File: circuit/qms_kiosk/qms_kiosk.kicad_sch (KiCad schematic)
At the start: 3 parts, among them U1 LCD2X16, U2 CEG003400, U3 ESP32-CAM

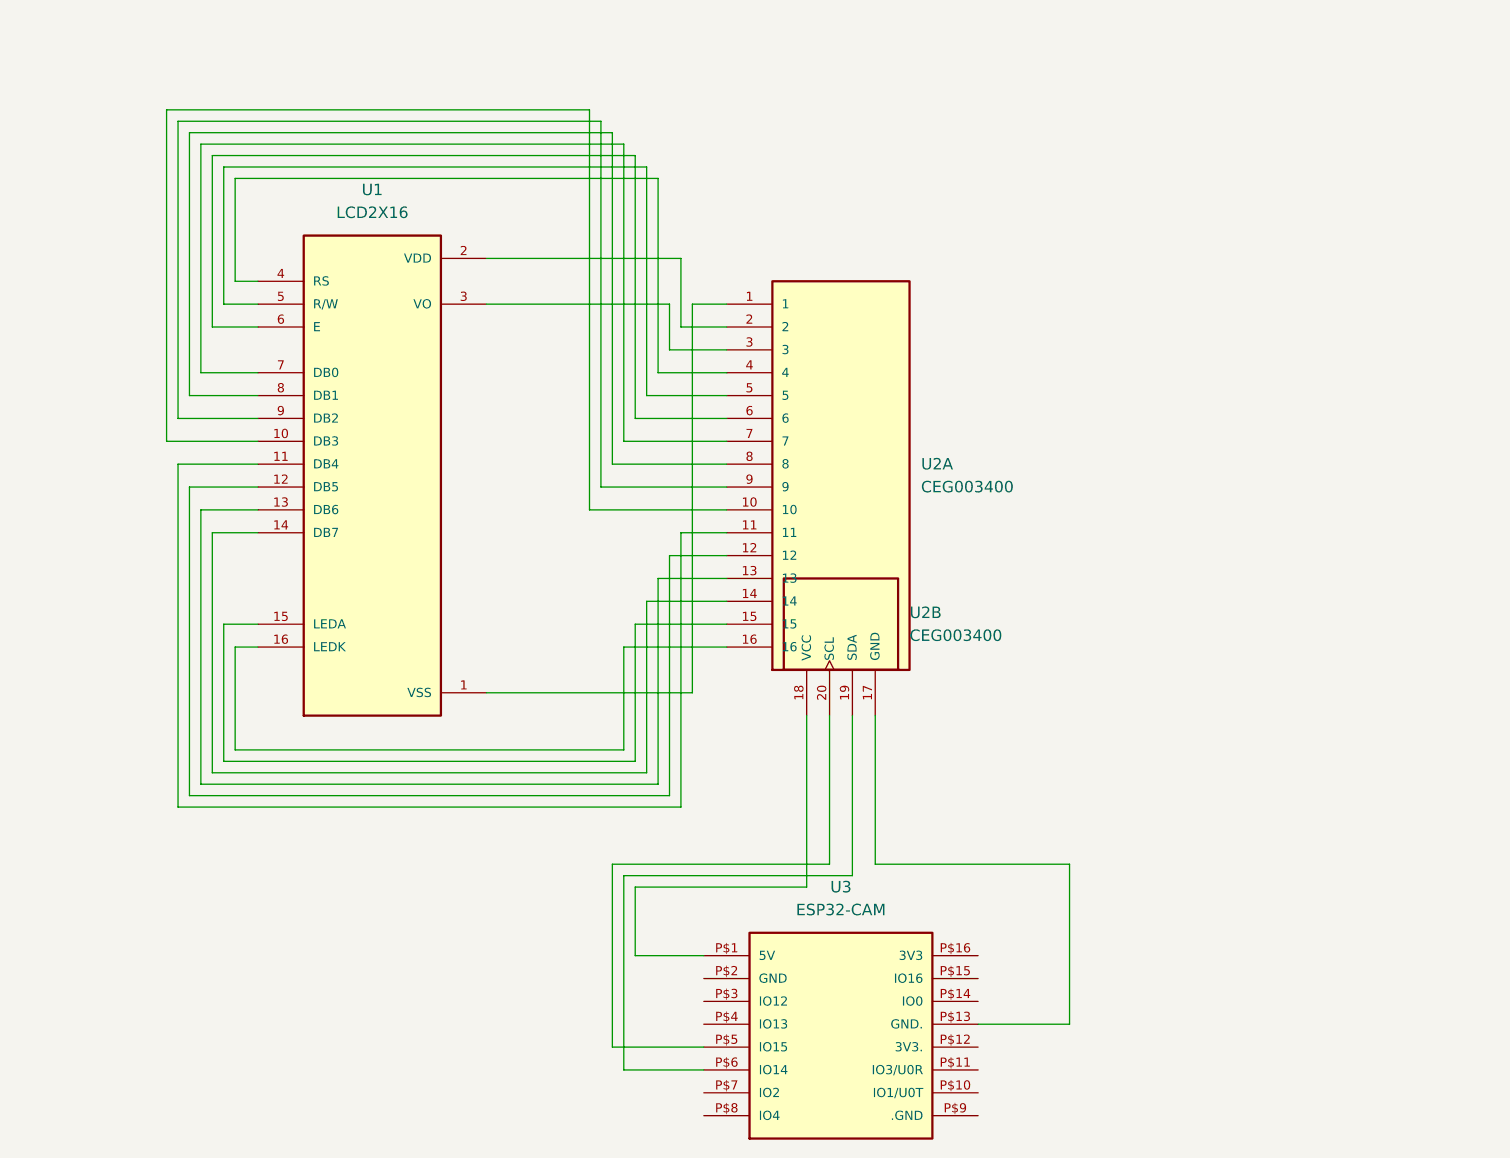
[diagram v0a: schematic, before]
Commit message: wip: Modified the Kiosk system schematic circuit.
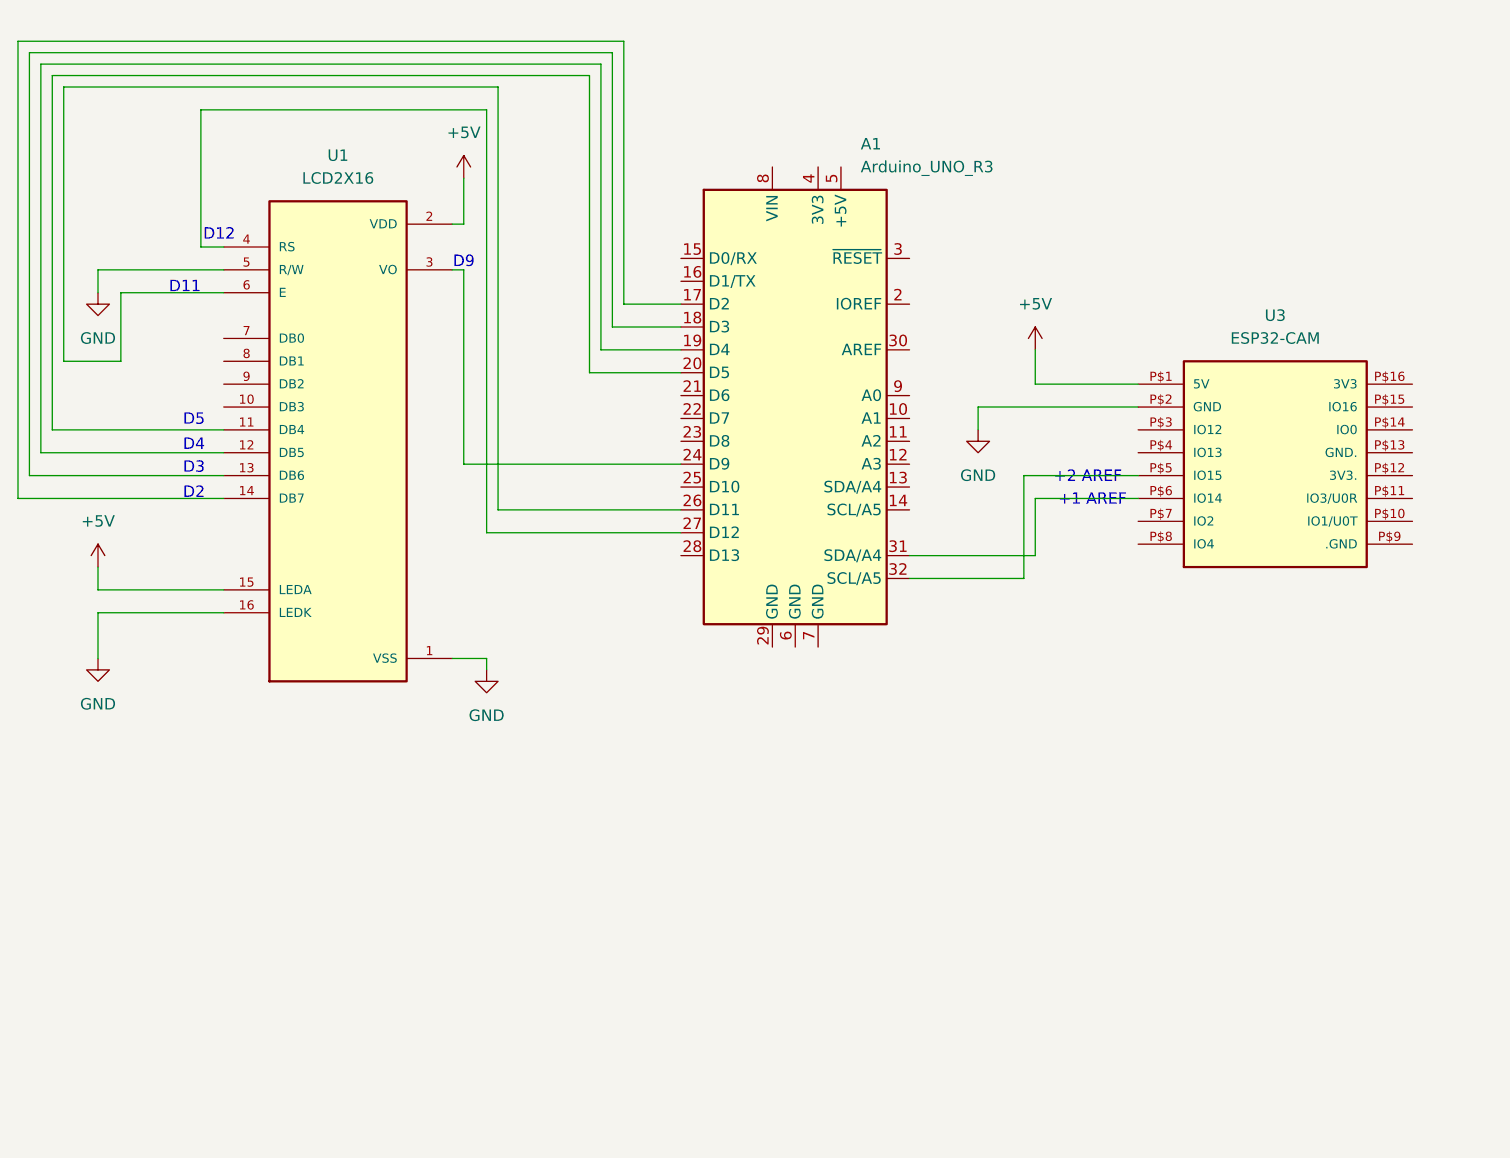
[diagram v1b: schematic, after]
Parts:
- removed U2: CEG003400, CEG003400:MODULE_CEG003400, symbol Board Module Port I2C for LCD:CEG003400
- added A1: Arduino_UNO_R3, Module:Arduino_UNO_R3, symbol MCU_Module:Arduino_UNO_R3
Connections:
- net GND: now reaches U1.1 (VSS)
- net GND: now also U1.16 (LEDK), U1.5 (R/W), U3.P$2 (GND)
- net at U1.11 (DB4): now also A1.20 (D5)
- net at U1.12 (DB5): now also A1.19 (D4)
- net at U1.13 (DB6): now also A1.18 (D3)
- net at U1.14 (DB7): now also A1.17 (D2)
- net +5V: now reaches U1.15 (LEDA)
- net +5V: now also U1.2 (VDD), U3.P$1 (5V)
- net at U1.3 (VO): now also A1.24 (D9)
- net at U1.4 (RS): now also A1.27 (D12)
- net at U1.6 (E): now also A1.26 (D11)
- net at U3.P$5 (IO15): now also A1.32 (SCL/A5)
- net at U3.P$6 (IO14): now also A1.31 (SDA/A4)
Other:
- note added: "+1 AREF"
- note added: "+2 AREF"
- note added: "D11"
- note added: "D12"
- note added: "D2"
- note added: "D3"
- note added: "D4"
- note added: "D5"
- note added: "D9"
- moved on the sheet: U1, U3

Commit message: wip: Update the pcb footprint of the components.
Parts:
- U1: footprint LCD2X16:LCD_LCD2X16 -> LCD 16x4(16x2) Display:LCD_LCD2X16
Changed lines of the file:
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@@
 			)
 		)
-		(property "Footprint" "LCD2X16:LCD_LCD2X16"
+		(property "Footprint" "LCD 16x4(16x2) Display:LCD_LCD2X16"
 			(at 107.95 72.39 0)
 			(effects

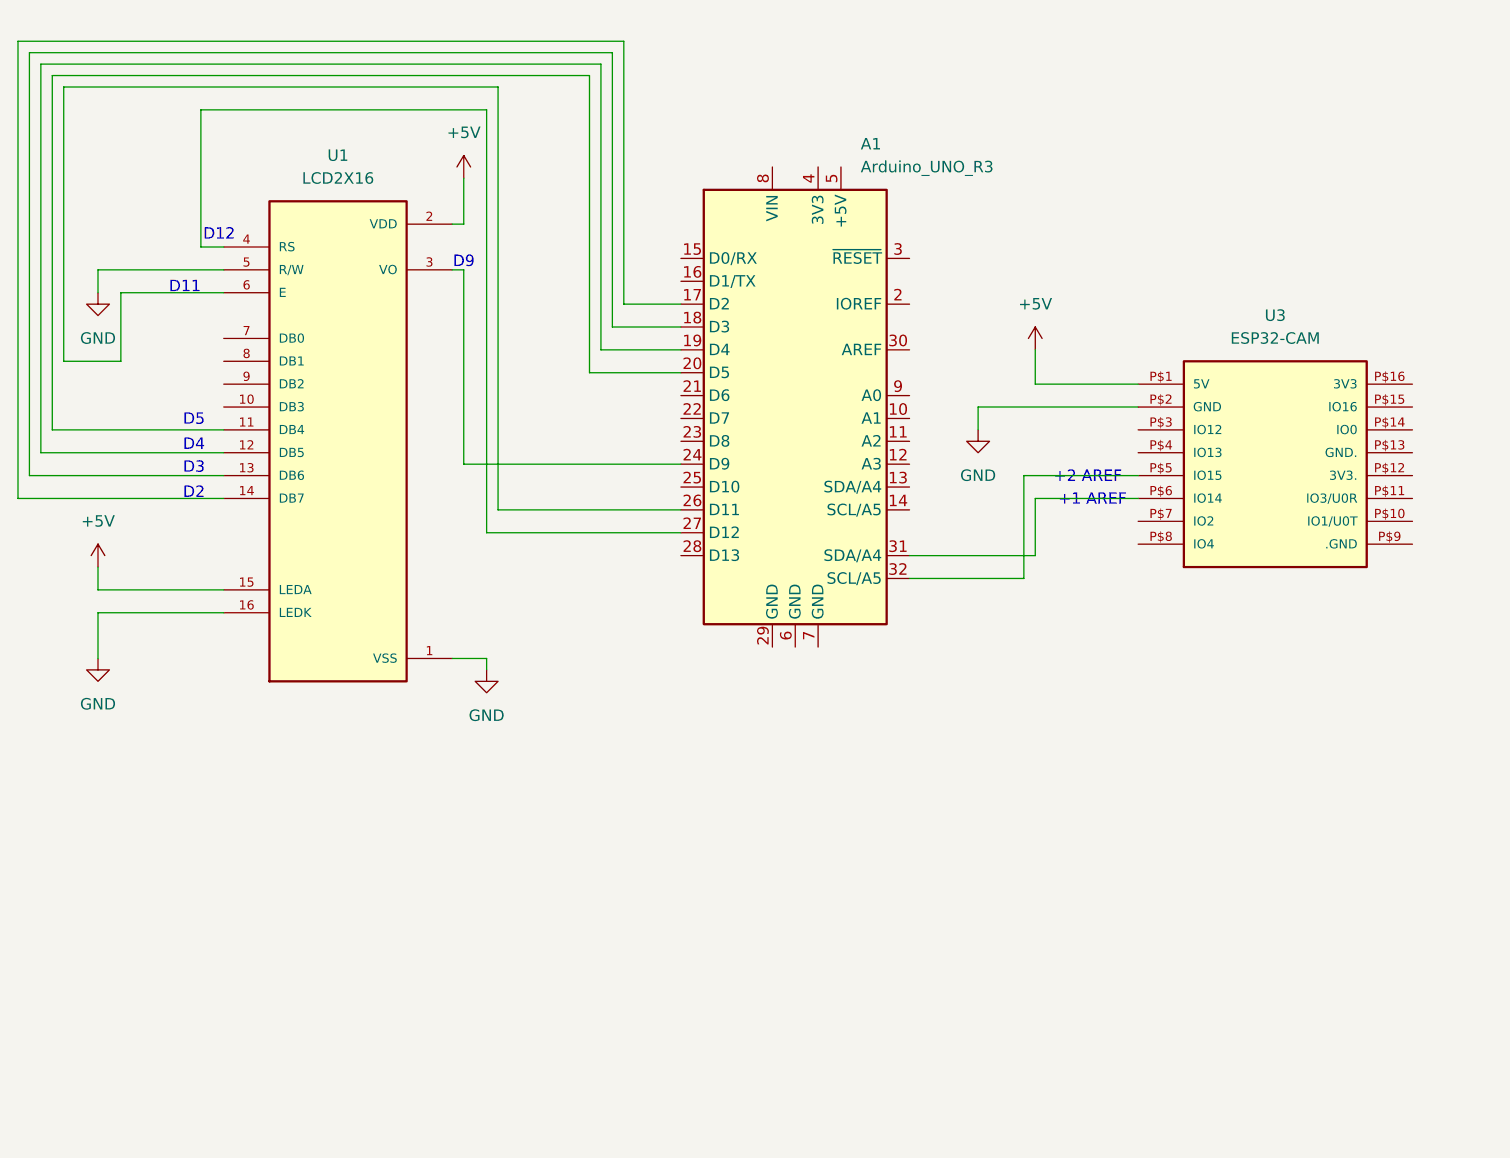
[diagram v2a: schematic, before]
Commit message: wip: First draft complete kiosk circuit.
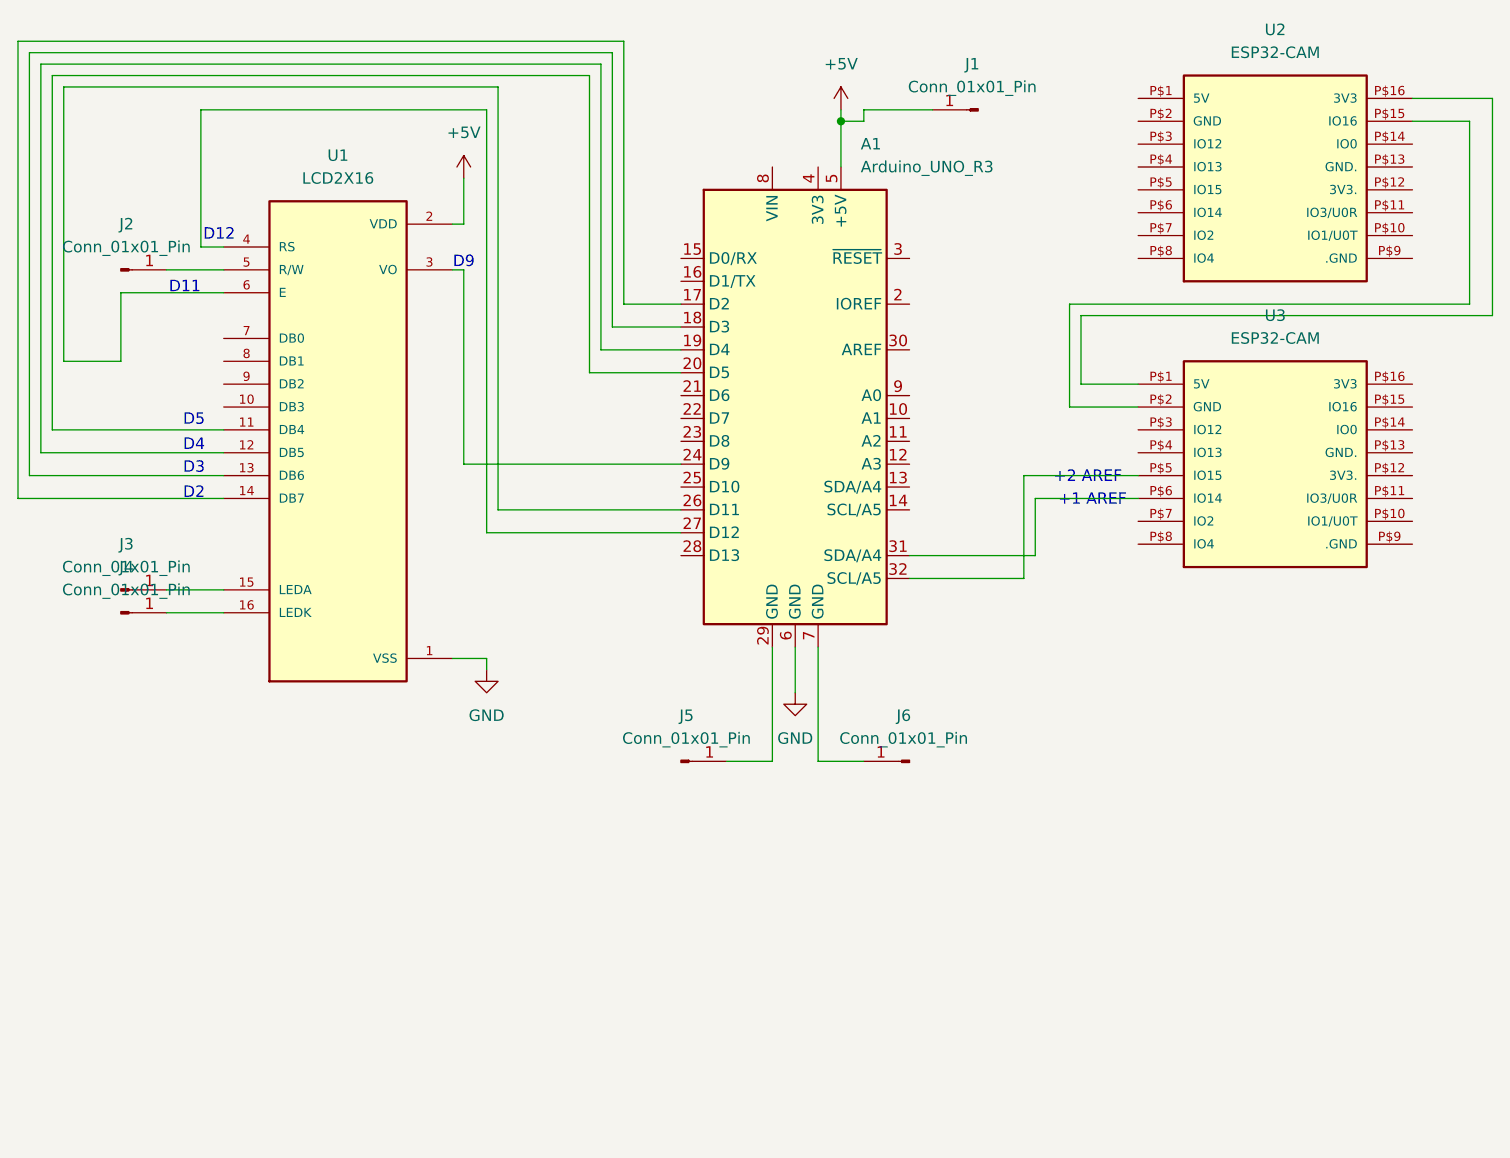
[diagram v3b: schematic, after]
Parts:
- added J1, J2, J3, J4, J5, J6: Conn_01x01_Pin, Connector_PinHeader_2.00mm:PinHeader_1x01_P2.00mm_Vertical, symbol Connector:Conn_01x01_Pin
- added U2: ESP32-CAM, ESP32-CAM:ESP32-CAM, symbol ESP32-CAM:ESP32-CAM
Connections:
- net +5V: now also A1.5 (+5V), J1.1 (Pin_1); no longer U1.15 (LEDA), U3.P$1 (5V)
- net GND: now also A1.6 (GND); no longer U1.16 (LEDK), U1.5 (R/W), U3.P$2 (GND)
- net at A1.29 (GND): now also J5.1 (Pin_1)
- net at A1.7 (GND): now also J6.1 (Pin_1)
- new net: J2.1 (Pin_1), U1.5 (R/W)
- new net: J4.1 (Pin_1), U1.16 (LEDK)
- new net: U2.P$16 (3V3), U3.P$1 (5V)
- new net: U2.P$15 (IO16), U3.P$2 (GND)
- new net: J3.1 (Pin_1), U1.15 (LEDA)
